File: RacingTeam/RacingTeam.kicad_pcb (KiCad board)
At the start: 4 copper layers, 104 x 92 mm, 77 parts, among them J1 BusIn, J2 Conn_01x01, J3 Conn_01x01, J4 Conn_01x01, J5 Conn_01x01, J6 PreCharge Relay Out, J7 AIROut, J8 Discharge Relay Out, J9 PCB OUT, Q1 TP0610T, Q2 2N7002, Q3 2N7002, Q4 2N7002, Q5 2N7002, Q6 TP0610T, Q7 2N7002, Q8 TP0610T, U1 LM311, U2 LM311, U3 4N35, U6 NE555D

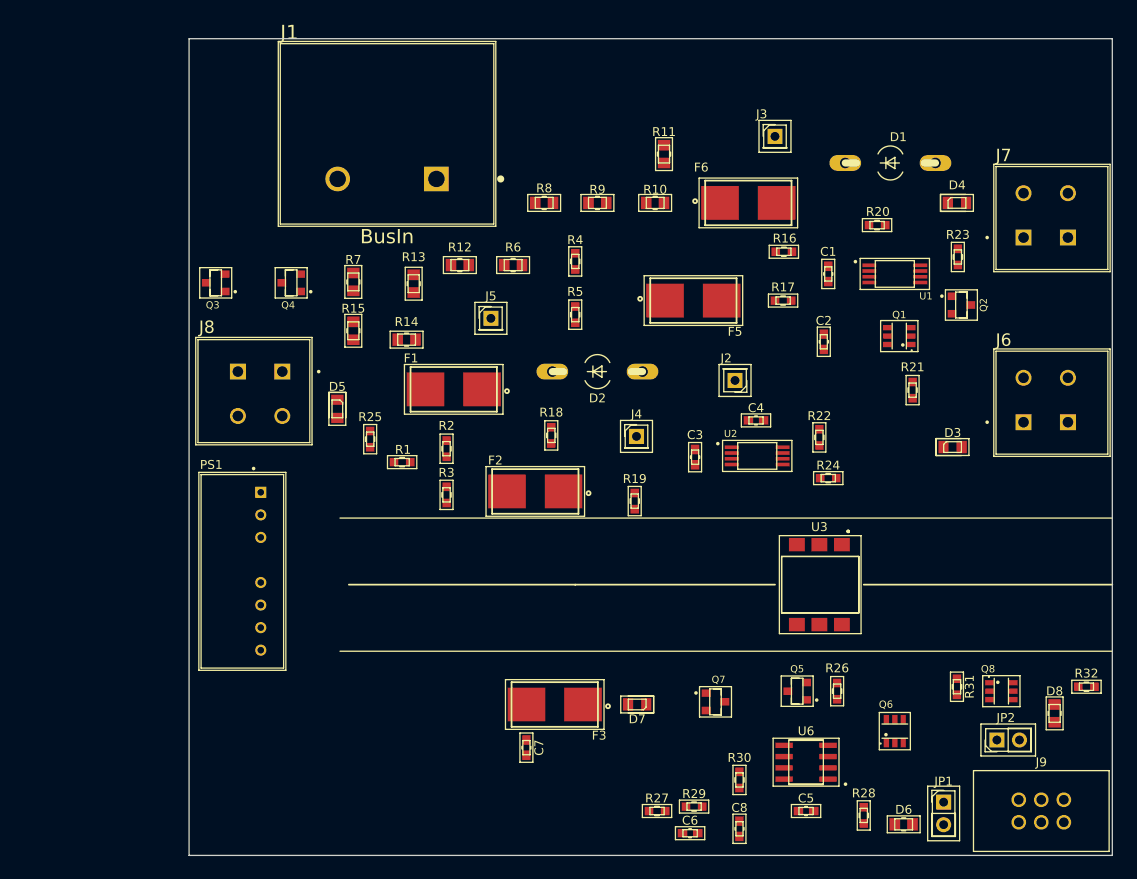
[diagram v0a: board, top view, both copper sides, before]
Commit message: Update FSAELogo.kicad_mod, GRC2022.mod, and 11 more files...
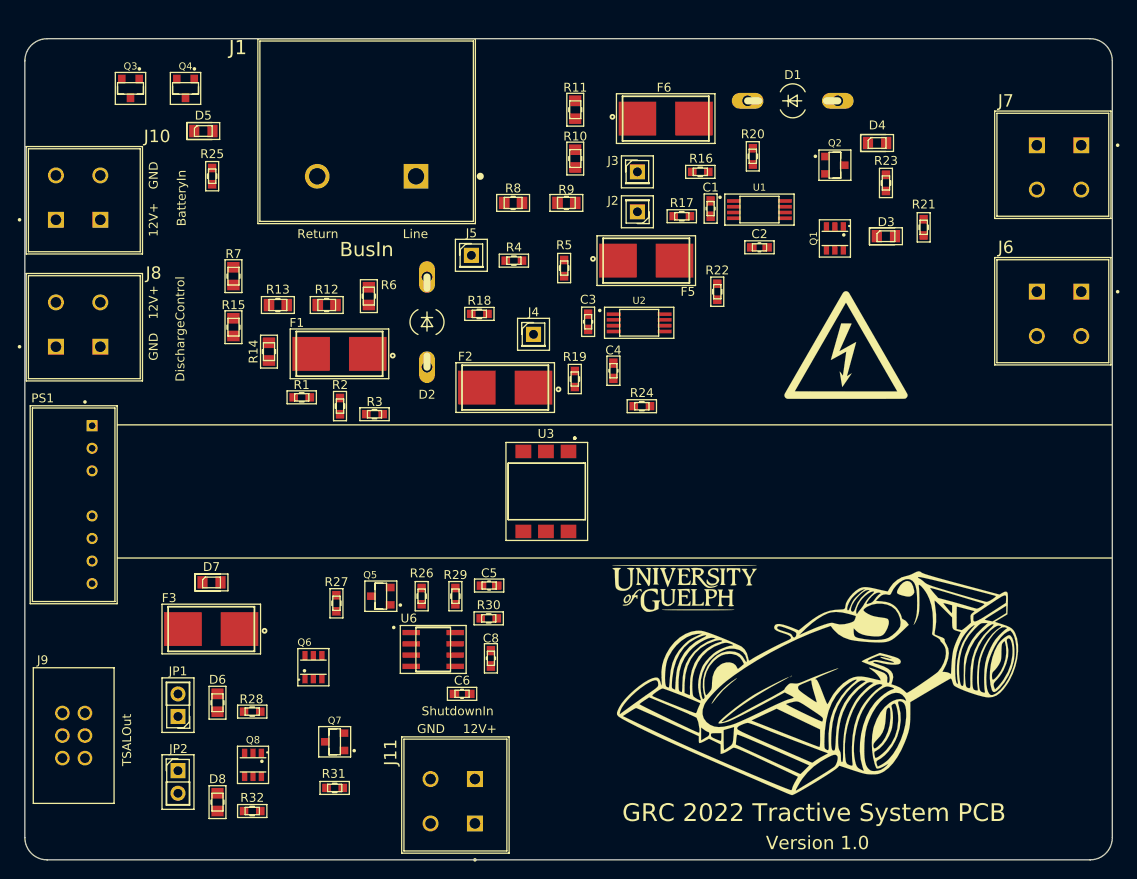
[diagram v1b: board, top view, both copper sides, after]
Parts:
- removed C7: C7, GRC2022:C_0603
- added G***: LOGO, Footprints:PCB, F.Cu at (198.8, 103.6)
- added G***: LOGO, Footprints:UofGLogo, F.Cu at (183.8, 93.0)
- added G***: LOGO, Footprints:HVLogo, F.Cu at (202.0, 65.5)
- added J10: BatteryIn, GRC2022:CUI_TBL001-500-02GY-2GY, F.Cu at (113.0, 51.4)
- added J11: ShutdownIn, GRC2022:CUI_TBL001-500-02GY-2GY, F.Cu at (160.2, 119.4)
- D1, D2, J6, J7, J8, R7: moved to F.Cu
- moved J9 109.3 mm to (115.0, 109.5), turned to 270 degrees
- moved R32 95.0 mm to (135.1, 118.0)
- moved D8 94.8 mm to (131.2, 117.0), turned to 90 degrees
- moved JP2 92.3 mm to (126.8, 113.5), turned to 0 degrees
- moved JP1 86.8 mm to (126.8, 107.3), turned to 180 degrees
- moved Q8 84.7 mm to (135.2, 112.8), turned to 270 degrees
- moved D6 78.5 mm to (131.2, 105.8), turned to 90 degrees
- moved R31 71.0 mm to (144.4, 115.4), turned to 180 degrees
- moved R28 69.9 mm to (135.1, 106.8), turned to 180 degrees
- moved Q6 65.9 mm to (142.0, 101.8)
- moved D7 49.9 mm to (130.5, 92.2), turned to 0 degrees
- moved Q5 48.1 mm to (149.6, 93.8)
- moved R26 48.0 mm to (154.2, 93.8)
- moved U6 43.9 mm to (155.5, 99.8), turned to 0 degrees
- moved C5 43.8 mm to (161.8, 92.6), turned to 180 degrees
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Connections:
- C5 pad 2: Shutdown- -> GLV+
- C6 pad 2: Shutdown- -> GLV+
- C8 pad 2: Shutdown- -> GLV+
- D7 pad 1: Shutdown- -> GLV+
- PS1 pad 7: Shutdown- -> GLV+
- Q5 pad 1: Shutdown- -> GLV+
- Q6 pad 3: Shutdown- -> GLV+
- Q7 pad 1: Shutdown- -> GLV+
- Q8 pad 3: Shutdown- -> GLV+
- R26 pad 2: Shutdown- -> GLV+
- R28 pad 2: Shutdown- -> GLV+
- R31 pad 1: Shutdown- -> GLV+
- R32 pad 2: Shutdown- -> GLV+
- U6 pad 1: Shutdown- -> GLV+
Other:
- board size 104 x 92 mm -> 122.5 x 92.5 mm
- board text added: "12V+"
- board text added: "BatteryIn"
- board text added: "DischargeControl"
- board text added: "GND"
- board text added: "GRC 2022 Tractive System PCB"
- board text added: "Line"
- board text added: "Return"
- board text added: "ShutdownIn"
- board text added: "TSALOut"
- board text added: "Version 1.0"
